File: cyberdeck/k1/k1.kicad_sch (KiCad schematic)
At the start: 70 parts, among them J1 Conn_01x20_MountingPin, J2 Conn_01x20_MountingPin, SW0 #0 ), SW1 #1 !, SW2 #2 @, SW3 #3 #, SW4 #4 $, SW5 #5 %, SW6 #6 ^, SW7 #7 &, SW8 #8 *, SW9 #9 (

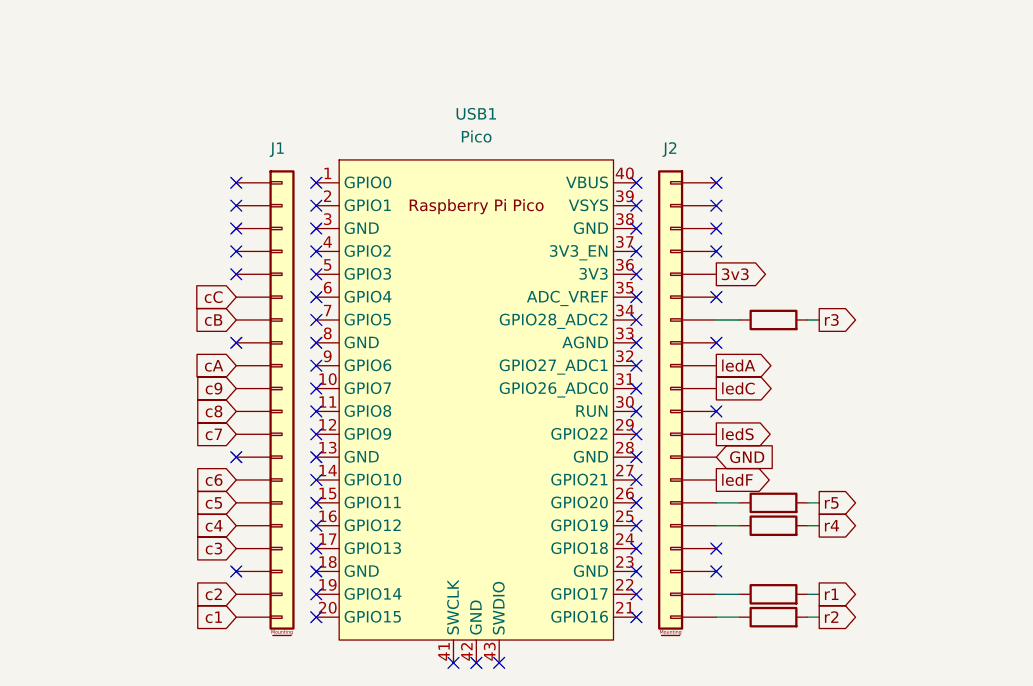
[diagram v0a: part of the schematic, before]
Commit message: posiblemente funcional
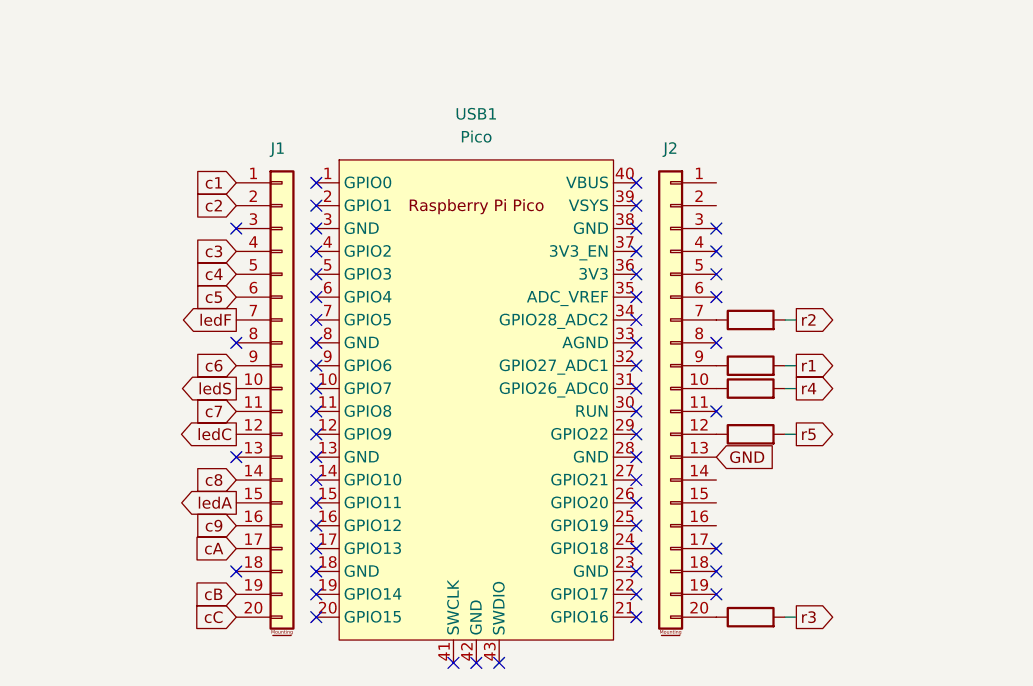
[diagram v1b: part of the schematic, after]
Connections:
- net c1: now also J1.1 (Pin_1); no longer J1.20 (Pin_20)
- net c2: now also J1.2 (Pin_2); no longer J1.19 (Pin_19)
- net c3: now also J1.4 (Pin_4); no longer J1.17 (Pin_17)
- net c4: now also J1.5 (Pin_5); no longer J1.16 (Pin_16)
- net c5: now also J1.6 (Pin_6); no longer J1.15 (Pin_15)
- net c6: now also J1.9 (Pin_9); no longer J1.14 (Pin_14)
- net c7: now also J1.11 (Pin_11); no longer J1.12 (Pin_12)
- net c8: now also J1.14 (Pin_14); no longer J1.11 (Pin_11)
- net c9: now also J1.16 (Pin_16); no longer J1.10 (Pin_10)
- net cA: now also J1.17 (Pin_17); no longer J1.9 (Pin_9)
- net cB: now also J1.19 (Pin_19); no longer J1.7 (Pin_7)
- net cC: now also J1.20 (Pin_20); no longer J1.6 (Pin_6)
- net ledA: now also J1.15 (Pin_15); no longer J2.9 (Pin_9)
- net ledC: now also J1.12 (Pin_12); no longer J2.10 (Pin_10)
- net ledF: now also J1.7 (Pin_7); no longer J2.14 (Pin_14)
- net ledS: now also J1.10 (Pin_10); no longer J2.12 (Pin_12)
- net at RR1.1: now also J2.9 (Pin_9); no longer J2.19 (Pin_19)
- net at RR3.1: now also J2.20 (Pin_20); no longer J2.7 (Pin_7)
- net at RR5.1: now also J2.12 (Pin_12); no longer J2.15 (Pin_15)
- net at RR2.1: now also J2.7 (Pin_7); no longer J2.20 (Pin_20)
- net at RR4.1: now also J2.10 (Pin_10); no longer J2.16 (Pin_16)
- net 3v3: no longer names the net of J2.5 (Pin_5)
- no-connect marks 60 -> 56
